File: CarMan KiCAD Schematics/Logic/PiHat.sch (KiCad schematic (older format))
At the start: 11 parts, among them J7 Conn_01x02_Male, U2 ISO1050DUB, U8 MCP2515-xSO, Y1 16MHz

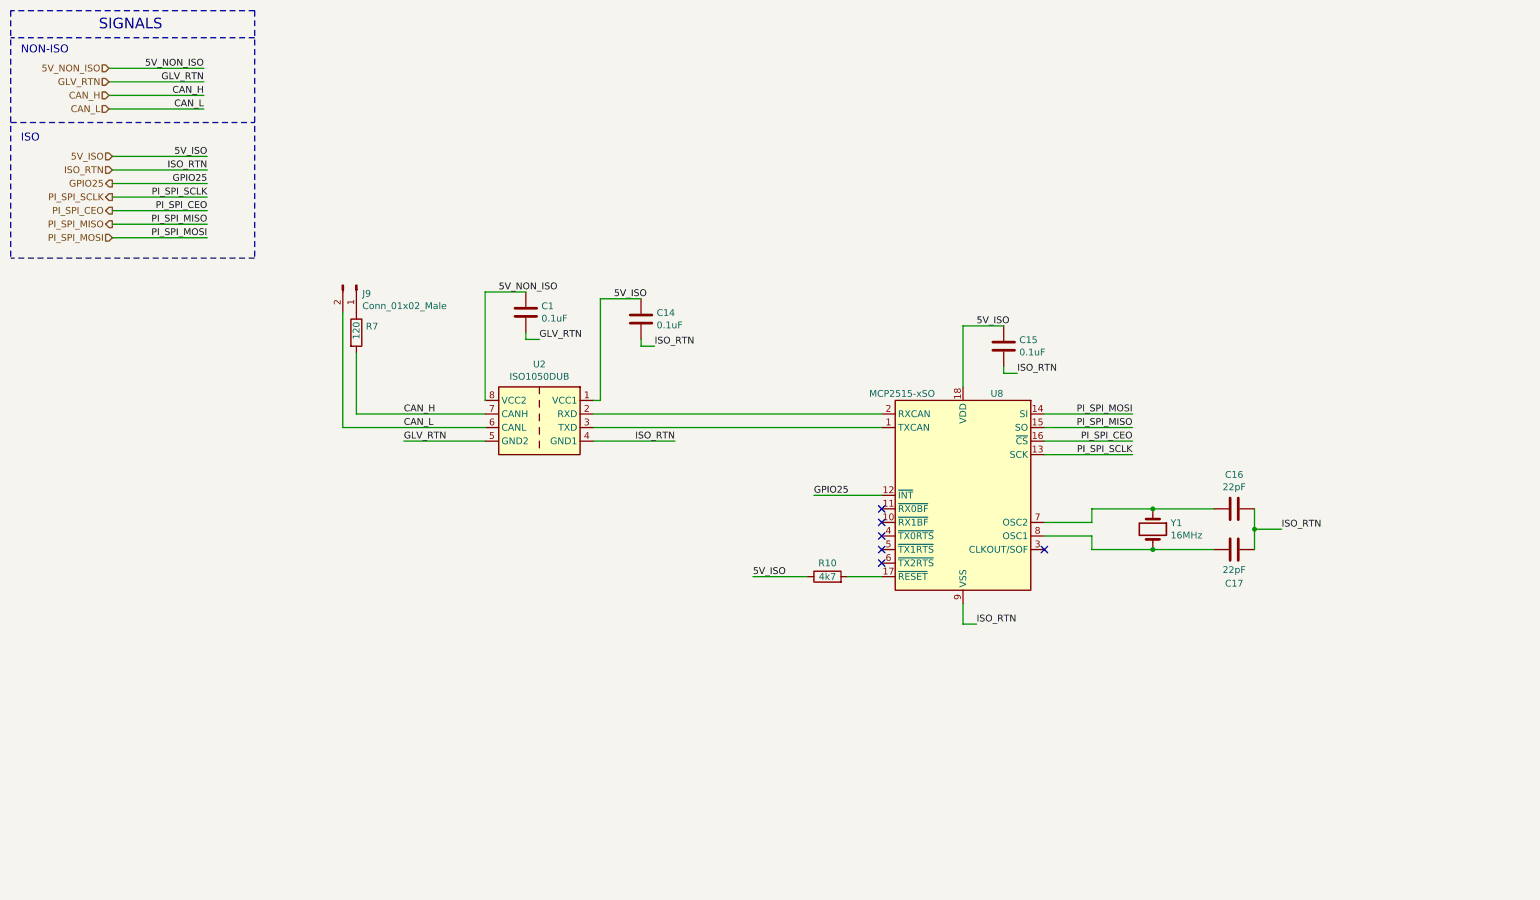
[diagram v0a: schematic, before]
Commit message: Logic Update
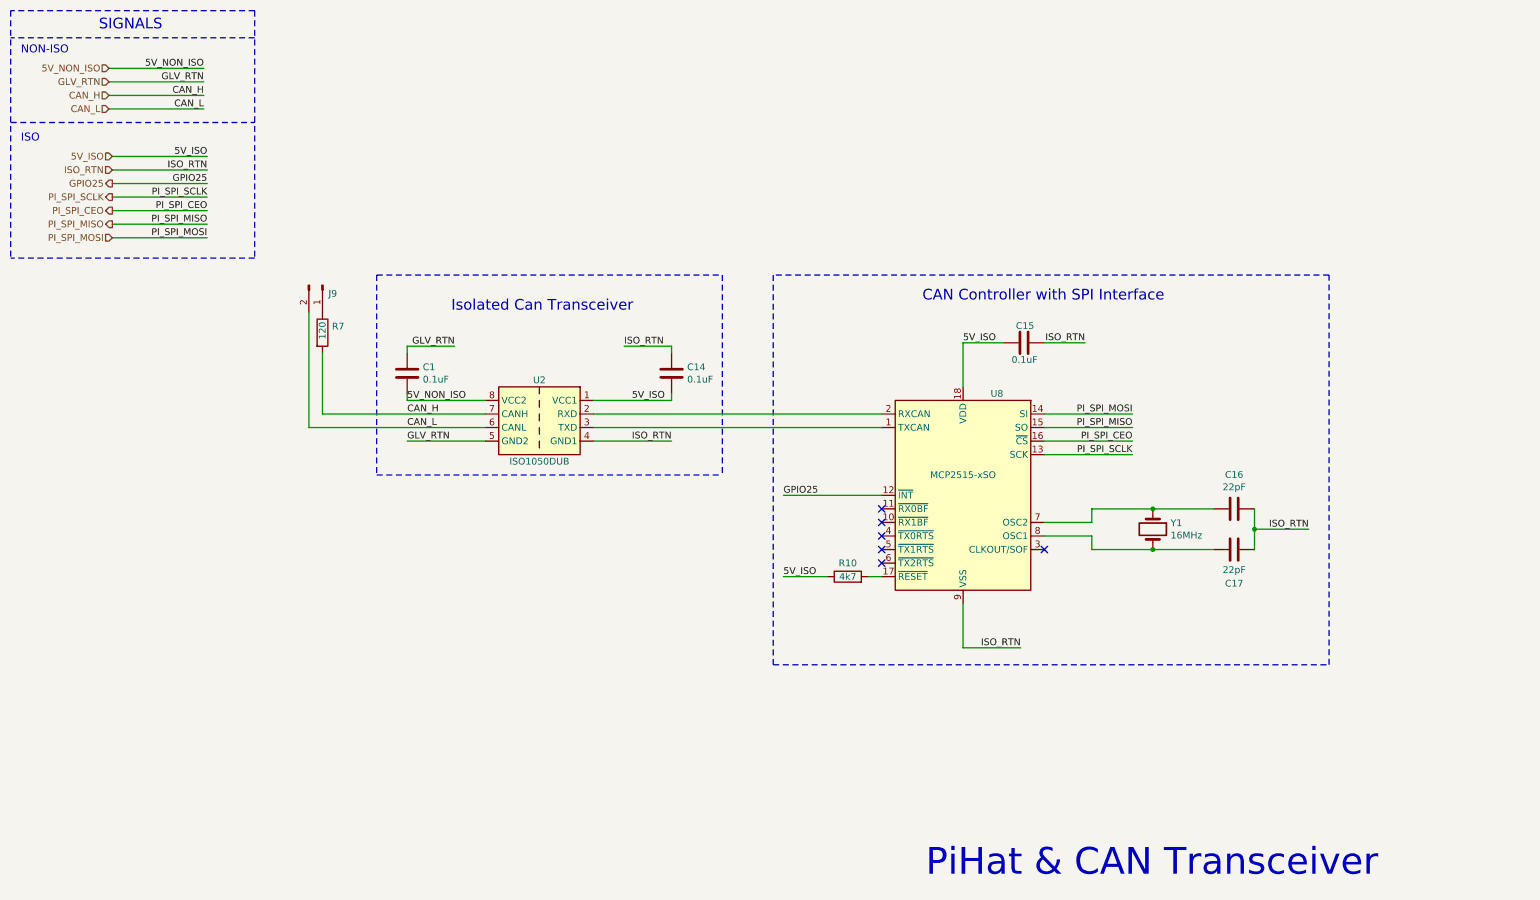
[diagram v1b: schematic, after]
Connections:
- net 5V_ISO: now also C14.2; no longer C14.1
- net 5V_NON_ISO: now also C1.2; no longer C1.1
- net GLV_RTN: now also C1.1; no longer C1.2
- net ISO_RTN: now also C14.1; no longer C14.2
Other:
- note added: "CAN Controller with SPI Interface"
- note added: "Isolated Can Transceiver"
- note added: "PiHat & CAN Transceiver"
- moved on the sheet: C1, C14, C15, J9, R10, R7
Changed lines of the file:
@@
 Text HLabel 1300 1625 0    50   Input ~ 0
 5V_ISO
-$Comp
-L Logic-rescue:MCP2515-xSO-Interface_CAN_LIN-Logic-rescue U8
-U 1 1 5F9A99EE
-P 7575 4125
-F 0 "U8" H 7325 4875 50  0000 C CNN
-F 1 "MCP2515-xSO" H 8025 4875 50  0000 C CNN
-F 2 "Package_SO:SOIC-18W_7.5x11.6mm_P1.27mm" H 7575 3225 50  0001 C CIN
-F 3 "http://ww1.microchip.com/downloads/en/DeviceDoc/21801e.pdf" H 7675 3325 50  0001 C CNN
-	1    7575 4125
-	-1   0    0    -1
-$EndComp
 Text HLabel 1300 1725 0    50   Input ~ 0
 ISO_RTN
-Text Label 3450 3525 0    50   ~ 0
+Text Label 3475 3525 0    50   ~ 0
 CAN_H
-Text Label 3450 3625 0    50   ~ 0
+Text Label 3475 3625 0    50   ~ 0
 CAN_L
 Text Label 2000 1625 2    50   ~ 0
@@
 L Logic-rescue:Conn_01x02_Male-Connector-Logic-rescue J7
 U 1 1 5F9AE3B8
-P 3100 2575
+P 2850 2575
 AR Path="/5F9AE3B8" Ref="J7"  Part="1"
 AR Path="/5F9A7CF0/5F9AE3B8" Ref="J9"  Part="1"
-F 0 "J9" V 3162 2619 50  0000 L CNN
-F 1 "Conn_01x02_Male" V 3253 2619 50  0000 L CNN
-F 2 "Connector_PinSocket_2.54mm:PinSocket_1x02_P2.54mm_Vertical" H 3100 2575 50  0001 C CNN
-F 3 "~" H 3100 2575 50  0001 C CNN
-	1    3100 2575
+F 0 "J9" V 2912 2619 50  0000 L CNN
+F 1 "Conn_01x02_Male" V 3050 1725 50  0001 L CNN
+F 2 "Connector_PinSocket_2.54mm:PinSocket_1x02_P2.54mm_Vertical" H 2850 2575 50  0001 C CNN
+F 3 "~" H 2850 2575 50  0001 C CNN
+	1    2850 2575
 	0    1    1    0
 $EndComp
@@
 L Logic-rescue:R-Device-Logic-rescue R7
 U 1 1 5F9AF7D2
-P 3100 2925
+P 2850 2925
 AR Path="/5F9AF7D2" Ref="R7"  Part="1"
 AR Path="/5F9A7CF0/5F9AF7D2" Ref="R7"  Part="1"
-F 0 "R7" H 3170 2971 50  0000 L CNN
-F 1 "120" V 3100 2875 50  0000 L CNN
-F 2 "Resistor_SMD:R_0805_2012Metric_Pad1.15x1.40mm_HandSolder" V 3030 2925 50  0001 C CNN
-F 3 "~" H 3100 2925 50  0001 C CNN
-	1    3100 2925
+F 0 "R7" H 2920 2971 50  0000 L CNN
+F 1 "120" V 2850 2875 50  0000 L CNN
+F 2 "Resistor_SMD:R_0805_2012Metric_Pad1.15x1.40mm_HandSolder" V 2780 2925 50  0001 C CNN
+F 3 "~" H 2850 2925 50  0001 C CNN
+	1    2850 2925
 	1    0    0    -1
 $EndComp
 Wire Wire Line
-	3000 2775 3000 3625
-Wire Wire Line
-	4900 2675 5200 2675
-$Comp
-L Logic-rescue:C-Device-Logic-rescue C14
-U 1 1 5F9B08F3
-P 5200 2825
-AR Path="/5F9B08F3" Ref="C14"  Part="1"
-AR Path="/5F9A7CF0/5F9B08F3" Ref="C14"  Part="1"
-F 0 "C14" H 5315 2871 50  0000 L CNN
-F 1 "0.1uF" H 5315 2780 50  0000 L CNN
-F 2 "Capacitor_SMD:C_0805_2012Metric_Pad1.15x1.40mm_HandSolder" H 5238 2675 50  0001 C CNN
-F 3 "~" H 5200 2825 50  0001 C CNN
-	1    5200 2825
-	1    0    0    -1
-$EndComp
-Wire Wire Line
-	5200 2975 5200 3025
-Wire Wire Line
-	5200 3025 5300 3025
-Text Label 5000 2675 0    50   ~ 0
-5V_ISO
-Text Label 5300 3025 0    50   ~ 0
-ISO_RTN
-Text Label 5450 3725 2    50   ~ 0
+	2750 2775 2750 3625
+Wire Wire Line
+	5425 3375 5425 3425
+Text Label 5075 3025 0    50   ~ 0
+ISO_RTN
+Text Label 5425 3725 2    50   ~ 0
 ISO_RTN
 NoConn ~ 8175 4525
-Text Label 7675 5075 0    50   ~ 0
-ISO_RTN
-Wire Wire Line
-	7575 4925 7575 5075
-Wire Wire Line
-	7575 5075 7675 5075
-Wire Wire Line
-	7575 3325 7575 2875
-Wire Wire Line
-	7575 2875 7875 2875
+Text Label 8000 5250 2    50   ~ 0
+ISO_RTN
+Wire Wire Line
+	7575 3000 7875 3000
 $Comp
 L Logic-rescue:C-Device-Logic-rescue C15
 U 1 1 5F9BD77C
-P 7875 3025
+P 8025 3000
 AR Path="/5F9BD77C" Ref="C15"  Part="1"
 AR Path="/5F9A7CF0/5F9BD77C" Ref="C15"  Part="1"
-F 0 "C15" H 7990 3071 50  0000 L CNN
-F 1 "0.1uF" H 7990 2980 50  0000 L CNN
-F 2 "Capacitor_SMD:C_0805_2012Metric_Pad1.15x1.40mm_HandSolder" H 7913 2875 50  0001 C CNN
-F 3 "~" H 7875 3025 50  0001 C CNN
-	1    7875 3025
-	1    0    0    -1
-$EndComp
-Wire Wire Line
-	7875 3175 7875 3225
-Wire Wire Line
-	7875 3225 7975 3225
-Text Label 7675 2875 0    50   ~ 0
-5V_ISO
-Text Label 7975 3225 0    50   ~ 0
-ISO_RTN
-Wire Wire Line
-	6975 4125 6475 4125
-Text Label 6475 4125 0    50   ~ 0
+F 0 "C15" V 8150 2925 50  0000 L CNN
+F 1 "0.1uF" V 7900 2900 50  0000 L CNN
+F 2 "Capacitor_SMD:C_0805_2012Metric_Pad1.15x1.40mm_HandSolder" H 8063 2850 50  0001 C CNN
+F 3 "~" H 8025 3000 50  0001 C CNN
+	1    8025 3000
+	0    -1   -1   0
+$EndComp
+Text Label 7575 3000 0    50   ~ 0
+5V_ISO
+Text Label 8475 3000 2    50   ~ 0
+ISO_RTN
+Text Label 6250 4125 0    50   ~ 0
 GPIO25
 NoConn ~ 6975 4225
@@
 L Logic-rescue:R-Device-Logic-rescue R10
 U 1 1 5F9C01C9
-P 6575 4725
+P 6725 4725
 AR Path="/5F9C01C9" Ref="R10"  Part="1"
 AR Path="/5F9A7CF0/5F9C01C9" Ref="R10"  Part="1"
-F 0 "R10" V 6675 4725 50  0000 C CNN
-F 1 "4k7" V 6575 4725 50  0000 C CNN
-F 2 "Resistor_SMD:R_0805_2012Metric_Pad1.15x1.40mm_HandSolder" V 6505 4725 50  0001 C CNN
-F 3 "~" H 6575 4725 50  0001 C CNN
-	1    6575 4725
+F 0 "R10" V 6825 4725 50  0000 C CNN
+F 1 "4k7" V 6725 4725 50  0000 C CNN
+F 2 "Resistor_SMD:R_0805_2012Metric_Pad1.15x1.40mm_HandSolder" V 6655 4725 50  0001 C CNN
+F 3 "~" H 6725 4725 50  0001 C CNN
+	1    6725 4725
 	0    -1   -1   0
 $EndComp
-Wire Wire Line
-	6725 4725 6975 4725
-Wire Wire Line
-	6425 4725 6025 4725
-Text Label 6025 4725 0    50   ~ 0
+Text Label 6250 4725 0    50   ~ 0
 5V_ISO
 Text Label 8825 3525 2    50   ~ 0
@@
 Wire Wire Line
 	9725 4225 9725 4375
-Wire Wire Line
-	9725 4375 9925 4375
 Connection ~ 9725 4375
 Wire Wire Line
 	9725 4375 9725 4525
-Text Label 9925 4375 0    50   ~ 0
-ISO_RTN
-Wire Wire Line
-	4900 3425 4850 3425
-Wire Wire Line
-	4900 2675 4900 3425
-Wire Wire Line
-	4050 2625 4350 2625
-$Comp
-L Logic-rescue:C-Device-Logic-rescue C1
-U 1 1 5FADAB07
-P 4350 2775
-AR Path="/5FADAB07" Ref="C1"  Part="1"
-AR Path="/5F9A7CF0/5FADAB07" Ref="C1"  Part="1"
-F 0 "C1" H 4465 2821 50  0000 L CNN
-F 1 "0.1uF" H 4465 2730 50  0000 L CNN
-F 2 "Capacitor_SMD:C_0805_2012Metric_Pad1.15x1.40mm_HandSolder" H 4388 2625 50  0001 C CNN
-F 3 "~" H 4350 2775 50  0001 C CNN
-	1    4350 2775
-	1    0    0    -1
-$EndComp
-Wire Wire Line
-	4350 2925 4350 2975
-Wire Wire Line
-	4350 2975 4450 2975
-Text Label 4150 2625 0    50   ~ 0
-5V_NON_ISO
-Text Label 4450 2975 0    50   ~ 0
+Text Label 10125 4375 2    50   ~ 0
+ISO_RTN
+Text Label 3825 3025 2    50   ~ 0
 GLV_RTN
 Text HLabel 1275 975  0    50   Input ~ 0
@@
 Text Label 1975 975  2    50   ~ 0
 5V_NON_ISO
-Wire Wire Line
-	4050 2625 4050 3425
 Text HLabel 1275 1075 0    50   Input ~ 0
 GLV_RTN
 Text Label 1975 1075 2    50   ~ 0
 GLV_RTN
-Text Label 3450 3725 0    50   ~ 0
+Text Label 3475 3725 0    50   ~ 0
 GLV_RTN
 Wire Wire Line
@@
 	1275 1075 1975 1075
 Wire Wire Line
-	3000 3625 4050 3625
-Wire Wire Line
-	3100 3075 3100 3525
-Wire Wire Line
-	3100 3525 4050 3525
-Wire Wire Line
-	3450 3725 4050 3725
+	2850 3075 2850 3525
 $Comp
 L Logic-rescue:ISO1050DUB-Interface_CAN_LIN-Logic-rescue U2
 U 1 1 5FAD2713
 P 4450 3525
-F 0 "U2" H 4450 3892 50  0000 C CNN
-F 1 "ISO1050DUB" H 4450 3801 50  0000 C CNN
+F 0 "U2" H 4450 3775 50  0000 C CNN
+F 1 "ISO1050DUB" H 4450 3175 50  0000 C CNN
 F 2 "Package_SO:SOP-8_6.62x9.15mm_P2.54mm" H 4450 3175 50  0001 C CIN
 F 3 "http://www.ti.com/lit/ds/symlink/iso1050.pdf" H 4450 3475 50  0001 C CNN
@@
 	-1   0    0    -1
 $EndComp
-Wire Wire Line
-	4850 3725 5450 3725
 Wire Wire Line
 	1300 1625 2000 1625
@@
 Wire Notes Line
 	2350 550  2350 2375
+Text Notes 7300 6950 0    197  ~ 0
+PiHat & CAN Transceiver
+Text Notes 3800 2775 0    79   ~ 0
+Isolated Can Transceiver
+Wire Wire Line
+	4850 3425 5425 3425
+Wire Wire Line
+	5425 3025 5425 3075
+Text Label 5375 3425 2    50   ~ 0
+5V_ISO
+Wire Wire Line
+	2850 3525 4050 3525
+Wire Wire Line
+	2750 3625 4050 3625
+Wire Wire Line
+	3475 3425 4050 3425
+Text Label 3475 3425 0    50   ~ 0
+5V_NON_ISO
+$Comp
+L Logic-rescue:C-Device-Logic-rescue C1
+U 1 1 5FADAB07
+P 3475 3225
+AR Path="/5FADAB07" Ref="C1"  Part="1"
+AR Path="/5F9A7CF0/5FADAB07" Ref="C1"  Part="1"
+F 0 "C1" H 3590 3271 50  0000 L CNN
+F 1 "0.1uF" H 3590 3180 50  0000 L CNN
+F 2 "Capacitor_SMD:C_0805_2012Metric_Pad1.15x1.40mm_HandSolder" H 3513 3075 50  0001 C CNN
+F 3 "~" H 3475 3225 50  0001 C CNN
+	1    3475 3225
+	1    0    0    -1
+$EndComp
+Wire Wire Line
+	3475 3375 3475 3425
+Wire Wire Line
+	3475 3025 3475 3075
+$Comp
+L Logic-rescue:C-Device-Logic-rescue C14
+U 1 1 5F9B08F3
+P 5425 3225
+AR Path="/5F9B08F3" Ref="C14"  Part="1"
+AR Path="/5F9A7CF0/5F9B08F3" Ref="C14"  Part="1"
+F 0 "C14" H 5540 3271 50  0000 L CNN
+F 1 "0.1uF" H 5540 3180 50  0000 L CNN
+F 2 "Capacitor_SMD:C_0805_2012Metric_Pad1.15x1.40mm_HandSolder" H 5463 3075 50  0001 C CNN
+F 3 "~" H 5425 3225 50  0001 C CNN
+	1    5425 3225
+	1    0    0    -1
+$EndComp
+Wire Wire Line
+	5075 3025 5425 3025
+Wire Wire Line
+	3475 3025 3825 3025
+Wire Wire Line
+	3475 3725 4050 3725
+Wire Wire Line
+	4850 3725 5425 3725
+Wire Notes Line
+	3250 3975 5800 3975
+Wire Wire Line
+	8175 3000 8475 3000
+$Comp
+L Logic-rescue:MCP2515-xSO-Interface_CAN_LIN-Logic-rescue U8
+U 1 1 5F9A99EE
+P 7575 4125
+F 0 "U8" H 7325 4875 50  0000 C CNN
+F 1 "MCP2515-xSO" H 7575 4275 50  0000 C CNN
+F 2 "Package_SO:SOIC-18W_7.5x11.6mm_P1.27mm" H 7575 3225 50  0001 C CIN
+F 3 "http://ww1.microchip.com/downloads/en/DeviceDoc/21801e.pdf" H 7675 3325 50  0001 C CNN
+	1    7575 4125
+	-1   0    0    -1
+$EndComp
+Wire Wire Line
+	7575 5250 8000 5250
+Wire Wire Line
+	7575 4925 7575 5250
+Wire Wire Line
+	7575 3000 7575 3325
+Wire Wire Line
+	6975 4725 6875 4725
+Wire Wire Line
+	6250 4725 6575 4725
+Wire Wire Line
+	6250 4125 6975 4125
+Wire Wire Line
+	9725 4375 10125 4375
+Wire Notes Line
+	6175 5375 10275 5375
+Wire Notes Line
+	10275 5375 10275 2500
+Wire Notes Line
+	10275 2500 6175 2500
+Wire Notes Line
+	6175 2500 6175 5375
+Text Notes 7275 2700 0    79   ~ 0
+CAN Controller with SPI Interface
+Wire Notes Line
+	5800 2500 5800 3975
+Wire Notes Line
+	3250 2500 5800 2500
+Wire Notes Line
+	3250 2500 3250 3975
 $EndSCHEMATC
